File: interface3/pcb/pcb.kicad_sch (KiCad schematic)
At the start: 27 parts, among them J1 Conn_Coaxial, T1 Murata 78602/8JC, U1 DS34LV86T, U2 DS34LV87T, U3 Pico_W

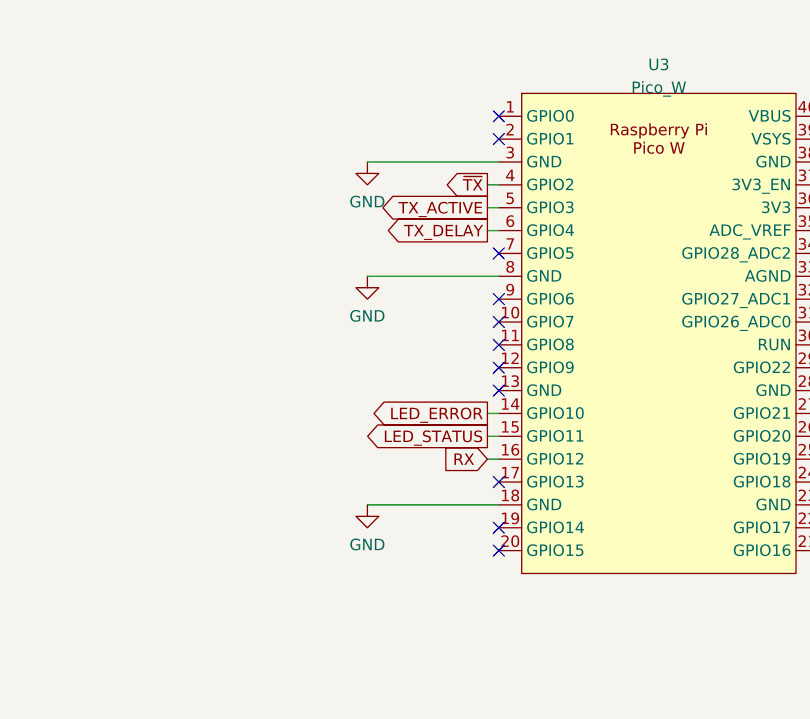
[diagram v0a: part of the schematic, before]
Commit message: some pcb work
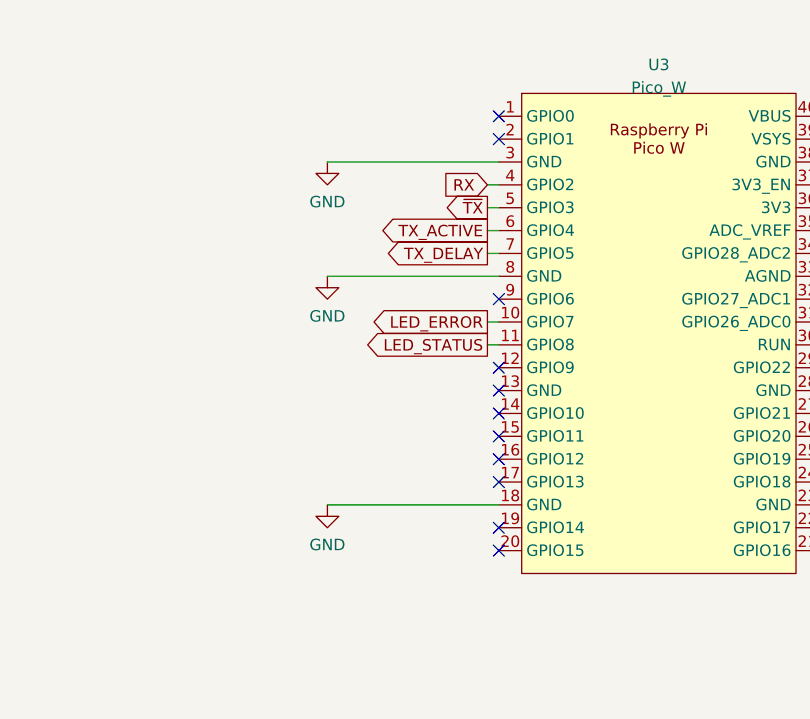
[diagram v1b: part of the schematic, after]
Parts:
- U3: footprint RPi_Pico:RPi_Pico_SMD_TH -> library:RPi_Pico_W_SMD_TH
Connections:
- net LED_ERROR: now also U3.10 (GPIO7); no longer U3.14 (GPIO10)
- net LED_STATUS: now also U3.11 (GPIO8); no longer U3.15 (GPIO11)
- net RX: now also U3.4 (GPIO2); no longer U3.16 (GPIO12)
- net TX_ACTIVE: now also U3.6 (GPIO4); no longer U3.5 (GPIO3)
- net TX_DELAY: now also U3.7 (GPIO5); no longer U3.6 (GPIO4)
- net ~{TX}: now also U3.5 (GPIO3); no longer U3.4 (GPIO2)
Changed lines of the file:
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@@
   (no_connect (at 123.19 71.755))
   (no_connect (at 123.19 97.155))
-  (no_connect (at 123.19 84.455))
+  (no_connect (at 123.19 107.315))
   (no_connect (at 346.71 207.01))
   (no_connect (at 158.75 86.995))
+  (no_connect (at 123.19 89.535))
   (no_connect (at 123.19 99.695))
   (no_connect (at 123.19 69.215))
@@
   (no_connect (at 289.56 180.34))
   (no_connect (at 353.06 180.34))
-  (no_connect (at 123.19 89.535))
+  (no_connect (at 123.19 102.235))
   (no_connect (at 158.75 94.615))
   (no_connect (at 158.75 114.935))
@@
   (no_connect (at 123.19 114.935))
   (no_connect (at 158.75 107.315))
-  (no_connect (at 123.19 92.075))
+  (no_connect (at 123.19 104.775))
   (no_connect (at 314.96 212.09))
   (no_connect (at 158.75 71.755))
-  (no_connect (at 123.19 94.615))
   (no_connect (at 158.75 104.775))
   (no_connect (at 158.75 102.235))
@@
     (stroke (width 0) (type default))
   )
-  (wire (pts (xy 108.585 74.295) (xy 123.19 74.295))
+  (wire (pts (xy 104.14 74.295) (xy 123.19 74.295))
     (stroke (width 0) (type default))
   )
@@
     (stroke (width 0) (type default))
   )
-  (wire (pts (xy 108.585 86.995) (xy 123.19 86.995))
+  (wire (pts (xy 104.14 86.995) (xy 123.19 86.995))
     (stroke (width 0) (type default))
   )
@@
     (stroke (width 0) (type default))
   )
-  (wire (pts (xy 121.92 107.315) (xy 123.19 107.315))
-    (stroke (width 0) (type default))
-  )
   (wire (pts (xy 289.56 217.17) (xy 289.56 209.55))
     (stroke (width 0) (type default))
@@
     (stroke (width 0) (type default))
   )
-  (wire (pts (xy 121.92 104.775) (xy 123.19 104.775))
+  (wire (pts (xy 121.92 92.075) (xy 123.19 92.075))
     (stroke (width 0) (type default))
   )
@@
     (stroke (width 0) (type default))
   )
-  (wire (pts (xy 108.585 112.395) (xy 123.19 112.395))
+  (wire (pts (xy 104.14 112.395) (xy 123.19 112.395))
     (stroke (width 0) (type default))
   )
@@
     (stroke (width 0) (type default))
   )
-  (wire (pts (xy 121.92 102.235) (xy 123.19 102.235))
+  (wire (pts (xy 121.92 94.615) (xy 123.19 94.615))
     (stroke (width 0) (type default))
   )
@@
   )
   (wire (pts (xy 302.26 107.95) (xy 304.8 107.95))
+    (stroke (width 0) (type default))
+  )
+  (wire (pts (xy 121.92 84.455) (xy 123.19 84.455))
     (stroke (width 0) (type default))
   )
@@
     (effects (font (size 2.0066 2.0066) italic) (justify left bottom))
   )
-  (global_label "RX" (shape input) (at 121.92 107.315 180)
+  (global_label "RX" (shape input) (at 121.92 76.835 180)
     (effects (font (size 1.27 1.27)) (justify right))
-    (property "Intersheetrefs" "${INTERSHEET_REFS}" (at 121.92 107.315 0)
-      (effects (font (size 1.27 1.27)) hide)
-    )
-  )
-  (global_label "TX_DELAY" (shape output) (at 121.92 81.915 180)
+    (property "Intersheetrefs" "${INTERSHEET_REFS}" (at 121.92 76.835 0)
+      (effects (font (size 1.27 1.27)) hide)
+    )
+  )
+  (global_label "TX_DELAY" (shape output) (at 121.92 84.455 180)
     (effects (font (size 1.27 1.27)) (justify right))
-    (property "Intersheetrefs" "${INTERSHEET_REFS}" (at 121.92 81.915 0)
+    (property "Intersheetrefs" "${INTERSHEET_REFS}" (at 121.92 84.455 0)
       (effects (font (size 1.27 1.27)) hide)
     )
@@
     )
   )
-  (global_label "TX_ACTIVE" (shape output) (at 121.92 79.375 180)
+  (global_label "TX_ACTIVE" (shape output) (at 121.92 81.915 180)
     (effects (font (size 1.27 1.27)) (justify right))
-    (property "Intersheetrefs" "${INTERSHEET_REFS}" (at 121.92 79.375 0)
+    (property "Intersheetrefs" "${INTERSHEET_REFS}" (at 121.92 81.915 0)
       (effects (font (size 1.27 1.27)) hide)
     )
@@
     )
   )
-  (global_label "LED_ERROR" (shape output) (at 121.92 102.235 180)
+  (global_label "LED_ERROR" (shape output) (at 121.92 92.075 180)
     (effects (font (size 1.27 1.27)) (justify right))
-    (property "Intersheetrefs" "${INTERSHEET_REFS}" (at 121.92 102.235 0)
+    (property "Intersheetrefs" "${INTERSHEET_REFS}" (at 121.92 92.075 0)
       (effects (font (size 1.27 1.27)) hide)
     )
@@
     )
   )
-  (global_label "LED_STATUS" (shape output) (at 121.92 104.775 180)
+  (global_label "LED_STATUS" (shape output) (at 121.92 94.615 180)
     (effects (font (size 1.27 1.27)) (justify right))
-    (property "Intersheetrefs" "${INTERSHEET_REFS}" (at 121.92 104.775 0)
+    (property "Intersheetrefs" "${INTERSHEET_REFS}" (at 121.92 94.615 0)
       (effects (font (size 1.27 1.27)) hide)
     )
@@
     )
   )
-  (global_label "~{TX}" (shape output) (at 121.92 76.835 180)
+  (global_label "~{TX}" (shape output) (at 121.92 79.375 180)
     (effects (font (size 1.27 1.27)) (justify right))
-    (property "Intersheetrefs" "${INTERSHEET_REFS}" (at 121.92 76.835 0)
+    (property "Intersheetrefs" "${INTERSHEET_REFS}" (at 121.92 79.375 0)
       (effects (font (size 1.27 1.27)) hide)
     )
@@
     )
   )
-  (symbol (lib_id "power:GND") (at 108.585 112.395 0) (unit 1)
+  (symbol (lib_id "power:GND") (at 104.14 112.395 0) (unit 1)
     (in_bom yes) (on_board yes) (dnp no) (fields_autoplaced)
-    (property "Reference" "#PWR04" (at 108.585 118.745 0)
-      (effects (font (size 1.27 1.27)) hide)
-    )
-    (property "Value" "GND" (at 108.585 116.84 0)
-      (effects (font (size 1.27 1.27)))
-    )
-    (property "Footprint" "" (at 108.585 112.395 0)
-      (effects (font (size 1.27 1.27)) hide)
-    )
-    (property "Datasheet" "" (at 108.585 112.395 0)
+    (property "Reference" "#PWR04" (at 104.14 118.745 0)
+      (effects (font (size 1.27 1.27)) hide)
+    )
+    (property "Value" "GND" (at 104.14 116.84 0)
+      (effects (font (size 1.27 1.27)))
+    )
+    (property "Footprint" "" (at 104.14 112.395 0)
+      (effects (font (size 1.27 1.27)) hide)
+    )
+    (property "Datasheet" "" (at 104.14 112.395 0)
       (effects (font (size 1.27 1.27)) hide)
     )
@@
     )
   )
-  (symbol (lib_id "power:GND") (at 108.585 86.995 0) (unit 1)
+  (symbol (lib_id "power:GND") (at 104.14 86.995 0) (unit 1)
     (in_bom yes) (on_board yes) (dnp no) (fields_autoplaced)
-    (property "Reference" "#PWR05" (at 108.585 93.345 0)
-      (effects (font (size 1.27 1.27)) hide)
-    )
-    (property "Value" "GND" (at 108.585 91.44 0)
-      (effects (font (size 1.27 1.27)))
-    )
-    (property "Footprint" "" (at 108.585 86.995 0)
-      (effects (font (size 1.27 1.27)) hide)
-    )
-    (property "Datasheet" "" (at 108.585 86.995 0)
+    (property "Reference" "#PWR05" (at 104.14 93.345 0)
+      (effects (font (size 1.27 1.27)) hide)
+    )
+    (property "Value" "GND" (at 104.14 91.44 0)
+      (effects (font (size 1.27 1.27)))
+    )
+    (property "Footprint" "" (at 104.14 86.995 0)
+      (effects (font (size 1.27 1.27)) hide)
+    )
+    (property "Datasheet" "" (at 104.14 86.995 0)
       (effects (font (size 1.27 1.27)) hide)
     )
@@
     )
   )
-  (symbol (lib_id "power:GND") (at 108.585 74.295 0) (unit 1)
+  (symbol (lib_id "power:GND") (at 104.14 74.295 0) (unit 1)
     (in_bom yes) (on_board yes) (dnp no) (fields_autoplaced)
-    (property "Reference" "#PWR06" (at 108.585 80.645 0)
-      (effects (font (size 1.27 1.27)) hide)
-    )
-    (property "Value" "GND" (at 108.585 78.74 0)
-      (effects (font (size 1.27 1.27)))
-    )
-    (property "Footprint" "" (at 108.585 74.295 0)
-      (effects (font (size 1.27 1.27)) hide)
-    )
-    (property "Datasheet" "" (at 108.585 74.295 0)
+    (property "Reference" "#PWR06" (at 104.14 80.645 0)
+      (effects (font (size 1.27 1.27)) hide)
+    )
+    (property "Value" "GND" (at 104.14 78.74 0)
+      (effects (font (size 1.27 1.27)))
+    )
+    (property "Footprint" "" (at 104.14 74.295 0)
+      (effects (font (size 1.27 1.27)) hide)
+    )
+    (property "Datasheet" "" (at 104.14 74.295 0)
       (effects (font (size 1.27 1.27)) hide)
     )
@@
       (effects (font (size 1.27 1.27)))
     )
-    (property "Footprint" "RPi_Pico:RPi_Pico_SMD_TH" (at 140.97 93.345 90)
-      (effects (font (size 1.27 1.27)) hide)
-    )
+    (property "Footprint" "library:RPi_Pico_W_SMD_TH" (at 140.97 93.345 90)
+      (effects (font (size 1.27 1.27)) hide)
+    )
